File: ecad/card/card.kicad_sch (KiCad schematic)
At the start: 138 parts, among them J1 Conn_01x03_Pin, J2 USB4105-GF-A, J3 10145226-0241N13LF, J4 Conn_01x03_Pin, SW1 SW_Push, SW2 SW_Push, U1 W25Q128JVS, U2 RP2350_80QFN, U3 MCP23017_SO, U4 NCP1117-3.3_SOT223, U5 MCP23017_SO, X1 ABM8-272-T3

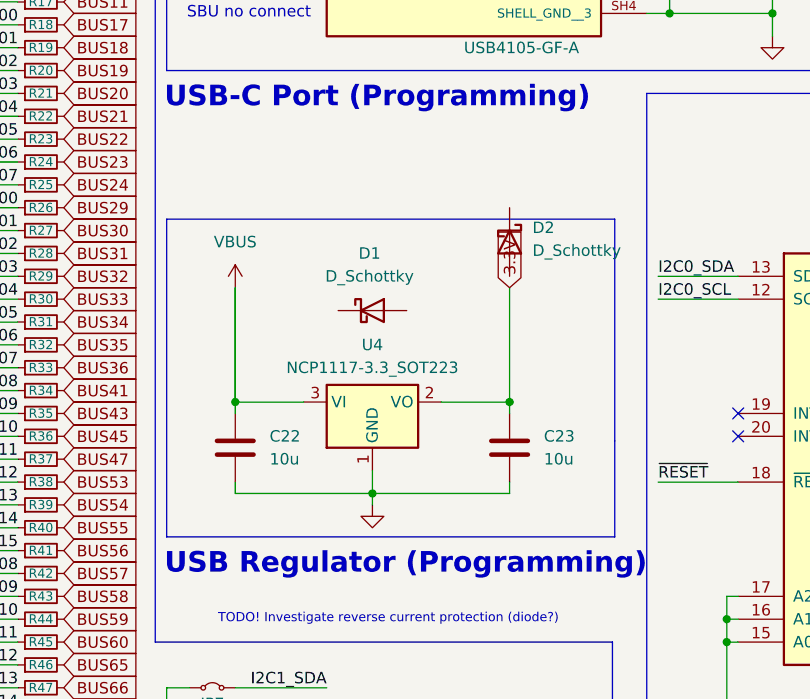
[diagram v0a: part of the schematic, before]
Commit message: Back panel changes
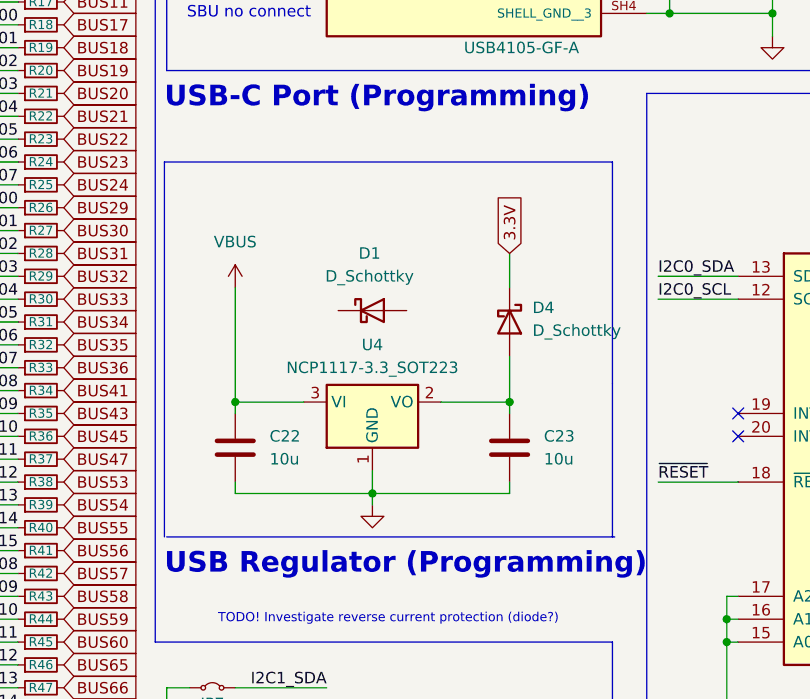
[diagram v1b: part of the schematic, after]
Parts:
- removed D2: D_Schottky, Diode_SMD:D_0402_1005Metric, symbol Device:D_Schottky
- added D4: D_Schottky, Diode_SMD:D_0402_1005Metric, symbol Device:D_Schottky
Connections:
- net 3.3V: now also D4.1 (K); no longer C23.1, U4.2 (VO)
- new net: C23.1, D4.2 (A), U4.2 (VO)
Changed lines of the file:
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@@
 	)
 	(junction
-		(at 204.47 132.08)
-		(diameter 0)
-		(color 0 0 0 0)
-	)
-	(junction
 		(at 30.48 74.93)
 		(diameter 0)
@@
 	)
 	(junction
+		(at 204.47 132.08)
+		(diameter 0)
+		(color 0 0 0 0)
+	)
+	(junction
 		(at 154.94 27.94)
 		(diameter 0)
@@
 	(polyline
 		(pts
-			(xy 216.154 136.398) (xy 216.154 147.066)
+			(xy 215.9 130.048) (xy 215.9 147.066)
 		)
 		(stroke
@@
 	(wire
 		(pts
-			(xy 204.47 119.38) (xy 204.47 132.08)
-		)
-		(stroke
-			(width 0)
-			(type default)
-		)
-	)
-	(wire
-		(pts
 			(xy 222.25 58.42) (xy 219.71 58.42)
 		)
@@
 	(polyline
 		(pts
-			(xy 216.154 111.76) (xy 216.154 136.398)
+			(xy 215.9 105.41) (xy 215.9 130.048)
 		)
 		(stroke
@@
 	(wire
 		(pts
+			(xy 204.47 115.57) (xy 204.47 119.38)
+		)
+		(stroke
+			(width 0)
+			(type default)
+		)
+	)
+	(wire
+		(pts
 			(xy 104.14 199.39) (xy 104.14 201.93)
 		)
@@
 	(polyline
 		(pts
-			(xy 166.37 147.066) (xy 166.37 111.76)
+			(xy 166.116 147.066) (xy 166.116 105.41)
 		)
 		(stroke
@@
 	(wire
 		(pts
-			(xy 173.99 119.38) (xy 173.99 132.08)
+			(xy 233.68 78.74) (xy 233.68 81.28)
 		)
 		(stroke
@@
 	(wire
 		(pts
-			(xy 233.68 78.74) (xy 233.68 81.28)
+			(xy 265.43 212.09) (xy 273.05 212.09)
 		)
 		(stroke
@@
 	(wire
 		(pts
-			(xy 265.43 212.09) (xy 273.05 212.09)
+			(xy 118.11 50.8) (xy 118.11 52.07)
 		)
 		(stroke
@@
 	(wire
 		(pts
-			(xy 118.11 50.8) (xy 118.11 52.07)
+			(xy 204.47 127) (xy 204.47 132.08)
 		)
 		(stroke
@@
 	(polyline
 		(pts
-			(xy 166.37 111.76) (xy 216.154 111.76)
+			(xy 166.116 105.41) (xy 215.9 105.41)
 		)
 		(stroke
@@
 	(global_label "3.3V"
 		(shape input)
-		(at 204.47 119.38 90)
+		(at 204.47 115.57 90)
 		(fields_autoplaced yes)
 		(effects
@@
 		)
 		(property "Intersheetrefs" "${INTERSHEET_REFS}"
-			(at 204.47 112.2824 90)
+			(at 204.47 108.4724 90)
 			(effects
 				(font
@@
 	)
 	(symbol
-		(lib_id "Device:D_Schottky")
-		(at 204.47 114.3 270)
-		(unit 1)
-		(exclude_from_sim no)
-		(in_bom yes)
-		(on_board yes)
-		(dnp no)
-		(fields_autoplaced yes)
-		(property "Reference" "D2"
-			(at 207.01 112.7124 90)
-			(effects
-				(font
-					(size 1.27 1.27)
-				)
-				(justify left)
-			)
-		)
-		(property "Value" "D_Schottky"
-			(at 207.01 115.2524 90)
-			(effects
-				(font
-					(size 1.27 1.27)
-				)
-				(justify left)
-			)
-		)
-		(property "Footprint" "Diode_SMD:D_0402_1005Metric"
-			(at 204.47 114.3 0)
-			(effects
-				(font
-					(size 1.27 1.27)
-				)
-				(hide yes)
-			)
-		)
-		(property "Datasheet" "~"
-			(at 204.47 114.3 0)
-			(effects
-				(font
-					(size 1.27 1.27)
-				)
-				(hide yes)
-			)
-		)
-		(property "Description" "Schottky diode"
-			(at 204.47 114.3 0)
-			(effects
-				(font
-					(size 1.27 1.27)
-				)
-				(hide yes)
-			)
-		)
-		(pin "1"
-		)
-		(pin "2"
-		)
-		(instances
-			(project "card"
-				(path "/9dd060f0-80a5-46f7-bd5a-b7a0ead0972f"
-					(reference "D2")
-					(unit 1)
-				)
-			)
-		)
-	)
-	(symbol
 		(lib_id "Device:R_Small")
 		(at 275.59 212.09 90)
@@
 					(unit 1)
 				)
+			)
+		)
+	)
+	(symbol
+		(lib_id "Device:D_Schottky")
+		(at 204.47 123.19 270)
+		(unit 1)
+		(exclude_from_sim no)
+		(in_bom yes)
+		(on_board yes)
+		(dnp no)
+		(fields_autoplaced yes)
+		(property "Reference" "D4"
+			(at 207.01 121.6024 90)
+			(effects
+				(font
+					(size 1.27 1.27)
+				)
+				(justify left)
+			)
+		)
+		(property "Value" "D_Schottky"
+			(at 207.01 124.1424 90)
+			(effects
+				(font
+					(size 1.27 1.27)
+				)
+				(justify left)
+			)
+		)
+		(property "Footprint" "Diode_SMD:D_0402_1005Metric"
+			(at 204.47 123.19 0)
+			(effects
+				(font
+					(size 1.27 1.27)
+				)
+				(hide yes)
+			)
+		)
+		(property "Datasheet" "~"
+			(at 204.47 123.19 0)
+			(effects
+				(font
+					(size 1.27 1.27)
+				)
+				(hide yes)
+			)
+		)
+		(property "Description" "Schottky diode"
+			(at 204.47 123.19 0)
+			(effects
+				(font
+					(size 1.27 1.27)
+				)
+				(hide yes)
+			)
+		)
+		(pin "1"
+		)
+		(pin "2"
+		)
+		(instances
+			(project "card"
+				(path "/9dd060f0-80a5-46f7-bd5a-b7a0ead0972f"
+					(reference "D4")
+					(unit 1)
+				)
